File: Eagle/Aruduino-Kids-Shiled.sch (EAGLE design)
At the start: 20 parts

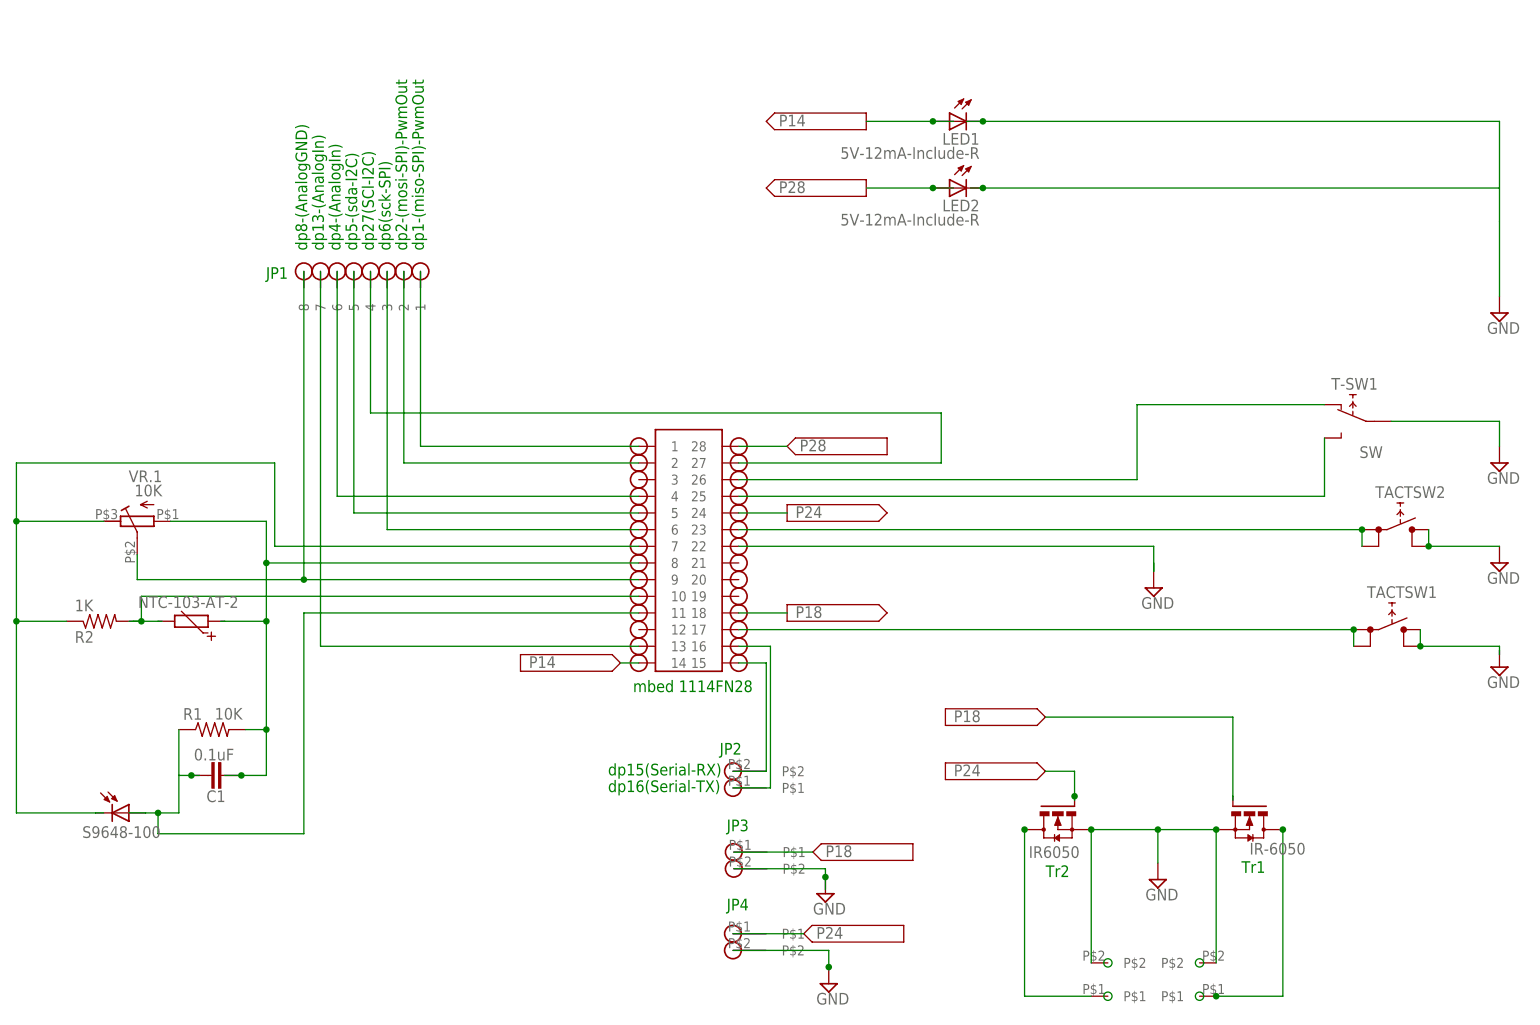
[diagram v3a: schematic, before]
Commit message: Final-P-ban
1st time
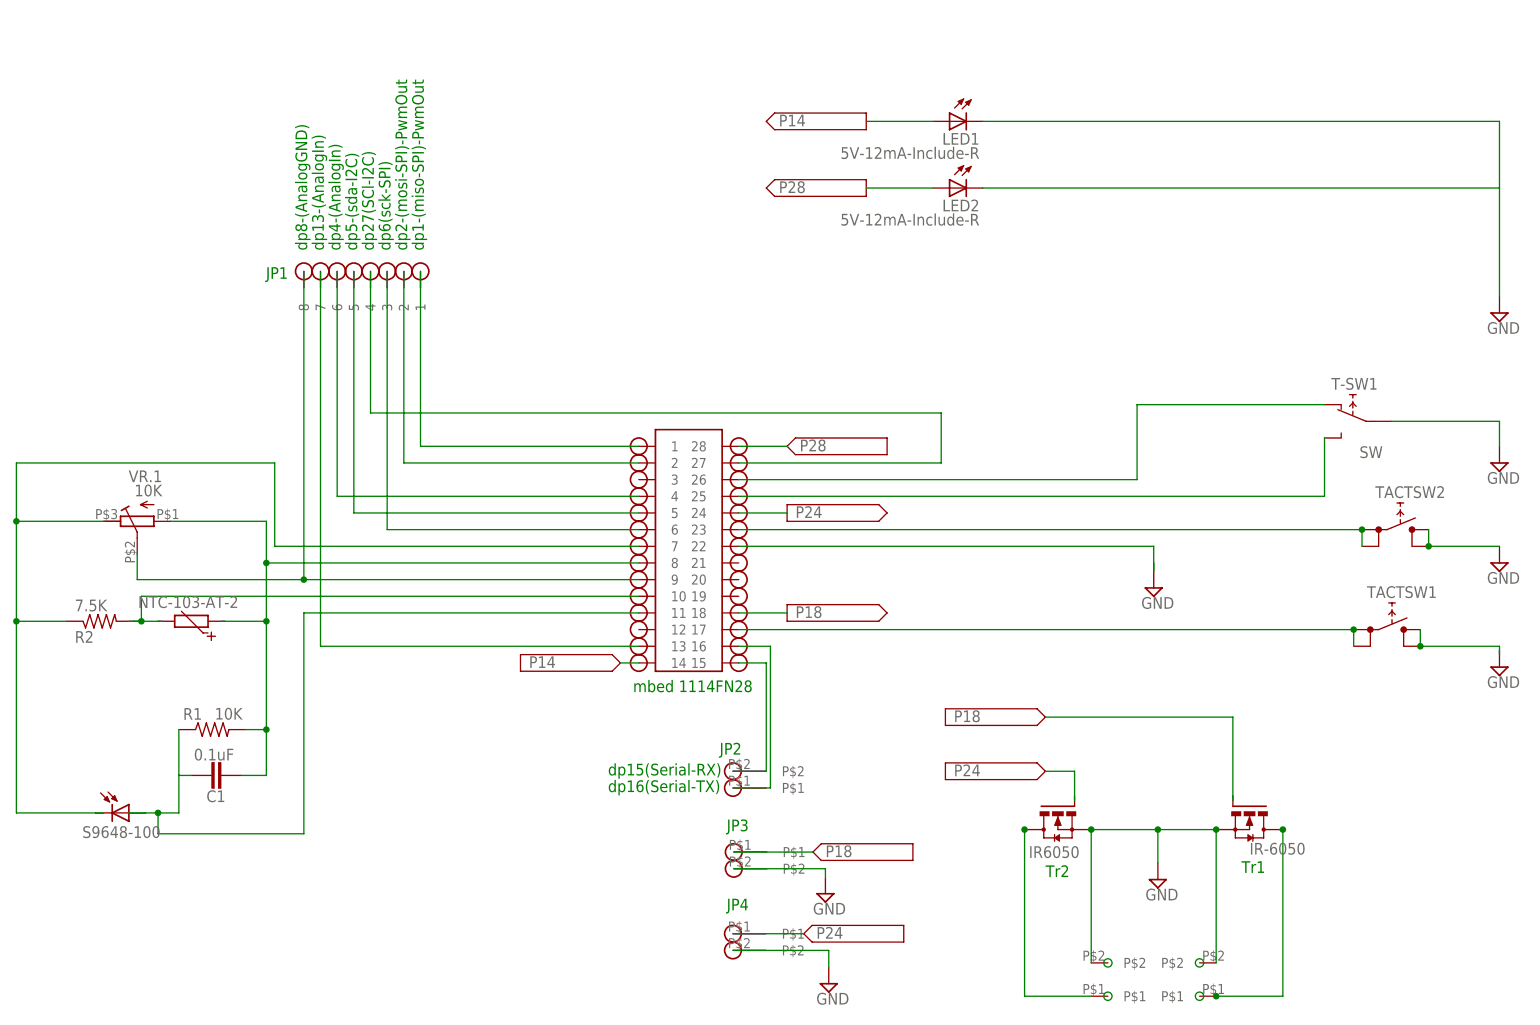
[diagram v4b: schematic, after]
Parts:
- R2: value 1K -> 7.5K
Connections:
- net GND renamed N$126
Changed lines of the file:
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@@
 <part name="SUPPLY12" library="supply2" deviceset="V&lt;--" device="" value="P18"/>
 <part name="SUPPLY13" library="supply2" deviceset="GND" device=""/>
-<part name="R2" library="Aruduino-Kids-Shiled" deviceset="R" device="" value="1K"/>
+<part name="R2" library="Aruduino-Kids-Shiled" deviceset="R" device="" value="7.5K"/>
 <part name="TACTSW2" library="Aruduino-Kids-Shiled" deviceset="TACT-SW" device=""/>
 <part name="TACTSW1" library="Aruduino-Kids-Shiled" deviceset="TACT-SW" device=""/>
@@
 </segment>
 <segment>
-<wire x1="203.2" y1="71.755" x2="200.025" y2="71.755" width="0.1524" layer="91"/>
 <pinref part="LED1" gate="G$1" pin="A"/>
 <wire x1="200.025" y1="71.755" x2="189.865" y2="71.755" width="0.1524" layer="91"/>
-<junction x="200.025" y="71.755"/>
 </segment>
 </net>
@@
 </segment>
 <segment>
-<wire x1="203.2" y1="61.595" x2="200.025" y2="61.595" width="0.1524" layer="91"/>
 <pinref part="LED2" gate="G$1" pin="A"/>
 <wire x1="200.025" y1="61.595" x2="189.865" y2="61.595" width="0.1524" layer="91"/>
-<junction x="200.025" y="61.595"/>
 </segment>
 </net>
@@
 <wire x1="98.425" y1="-20.955" x2="98.425" y2="-27.94" width="0.1524" layer="91"/>
 <junction x="98.425" y="-20.955"/>
-<wire x1="92.075" y1="-27.94" x2="94.615" y2="-27.94" width="0.1524" layer="91"/>
 <pinref part="C1" gate="G$1" pin="1"/>
 <wire x1="94.615" y1="-27.94" x2="98.425" y2="-27.94" width="0.1524" layer="91"/>
-<junction x="94.615" y="-27.94"/>
 <wire x1="91.44" y1="-4.445" x2="92.075" y2="-4.445" width="0.1524" layer="91"/>
 <wire x1="92.075" y1="-4.445" x2="98.425" y2="-4.445" width="0.1524" layer="91"/>
@@
 </segment>
 </net>
-<net name="GND" class="0">
+<net name="N$126" class="0">
 <segment>
 <pinref part="SUPPLY3" gate="GND" pin="GND"/>
@@
 </segment>
 <segment>
-<wire x1="286.385" y1="45.085" x2="286.385" y2="56.515" width="0.1524" layer="91"/>
+<wire x1="286.385" y1="45.085" x2="286.385" y2="61.595" width="0.1524" layer="91"/>
 <pinref part="SUPPLY9" gate="GND" pin="GND"/>
 <wire x1="286.385" y1="61.595" x2="286.385" y2="71.755" width="0.1524" layer="91"/>
-<wire x1="205.105" y1="71.755" x2="207.645" y2="71.755" width="0.1524" layer="91"/>
 <wire x1="207.645" y1="71.755" x2="286.385" y2="71.755" width="0.1524" layer="91"/>
-<wire x1="205.74" y1="61.595" x2="207.645" y2="61.595" width="0.1524" layer="91"/>
+<pinref part="LED1" gate="G$1" pin="C"/>
+<pinref part="LED2" gate="G$1" pin="C"/>
 <wire x1="207.645" y1="61.595" x2="286.385" y2="61.595" width="0.1524" layer="91"/>
-<wire x1="286.385" y1="61.595" x2="286.385" y2="56.515" width="0.1524" layer="91"/>
-<pinref part="LED1" gate="G$1" pin="C"/>
-<junction x="207.645" y="71.755"/>
-<pinref part="LED2" gate="G$1" pin="C"/>
-<junction x="207.645" y="61.595"/>
 </segment>
 <segment>
@@
 <wire x1="184.15" y1="-54.61" x2="184.15" y2="-57.15" width="0.1524" layer="91"/>
 <pinref part="SUPPLY10" gate="GND" pin="GND"/>
-<junction x="184.15" y="-57.15"/>
 <pinref part="U$9" gate="G$1" pin="P$2"/>
 </segment>
@@
 <wire x1="183.642" y1="-42.164" x2="183.642" y2="-43.434" width="0.1524" layer="91"/>
 <pinref part="SUPPLY13" gate="GND" pin="GND"/>
-<wire x1="183.642" y1="-43.434" x2="183.642" y2="-45.339" width="0.1524" layer="91"/>
-<junction x="183.642" y="-43.434"/>
 </segment>
 </net>
@@
 <wire x1="221.615" y1="-27.305" x2="217.17" y2="-27.305" width="0.1524" layer="91"/>
 <pinref part="U$5" gate="G$1" pin="G"/>
-<junction x="221.615" y="-31.115"/>
 </segment>
 <segment>
@@
 <wire x1="81.915" y1="-36.83" x2="81.915" y2="-33.655" width="0.1524" layer="91"/>
 <junction x="81.915" y="-33.655"/>
-<wire x1="88.265" y1="-27.94" x2="86.995" y2="-27.94" width="0.1524" layer="91"/>
 <pinref part="C1" gate="G$1" pin="2"/>
 <wire x1="86.995" y1="-27.94" x2="85.09" y2="-27.94" width="0.1524" layer="91"/>
-<junction x="86.995" y="-27.94"/>
 <pinref part="U$1" gate="G$1" pin="11"/>
 </segment>
@@
 </sheet>
 </sheets>
+<errors>
+</errors>
 </schematic>
 </drawing>

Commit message: Test-Sample-Build
Jet-PCB
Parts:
- LED1: value 5V-12mA-Include-R -> I-06245-R
- LED2: value 5V-12mA-Include-R -> I-06245-G
- T-SW1: value SW -> P-00300
- TACTSW1: value (none) -> P-03646-B
- TACTSW2: value (none) -> P-03646-R
- TB1, TB2: value 2A -> P-01306
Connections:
- net N$4 renamed 3.3V
- removed net N$126: LED1.C, LED2.C, T-SW1.2COM, TACTSW1.2, TACTSW1.4, TACTSW2.2, TACTSW2.4, TB1.P$2, TB2.P$2, U$1.22, U$10.P$2, U$4.S, U$5.S, U$9.P$2
- removed net N$6: 0-50C.1, C1.1, R1.2, U$1.8, VR.1.A
- new net A-GND: 0-50C.1, C1.1, R1.2, U$1.8, U$3.8, VR.1.A
- new net GND: LED1.C, LED2.C, T-SW1.2COM, TACTSW1.2, TACTSW1.4, TACTSW2.2, TACTSW2.4, TB1.P2, TB2.P2, U$1.22, U$10.P2, U$4.S, U$5.S, U$9.P2
- net N$21: now also TB2.P1; no longer TB2.P$1
- net N$22: now also TB1.P1; no longer TB1.P$1
- net N$26: now also U$6.P1; no longer U$6.P$1
- net N$27: now also U$6.P2; no longer U$6.P$2
- net N$8: no longer U$3.8
- net P18: now also U$10.P1; no longer U$10.P$1
- net P24: now also U$9.P1; no longer U$9.P$1
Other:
- note added: "C-03785"
- note added: "C-05779 (TP2,TP3,TP4)"
- note added: "I-02426"
- note added: "P-01306"
- note added: "P-06113"
- note added: "P-06165"
- note added: "P-07258"
- note added: "P1"
- note added: "P2"
- note added: "R-25103"
- note added: "R-25752"
- note added: "TP1"
- note added: "TP2"
- note added: "TP3"
- note added: "TP4"
- note removed: "JP1"
- note removed: "JP2"
- note removed: "JP3"
- note removed: "JP4"
- moved on the sheet: C1, LED1, LED2, R1, R2, T-SW1, TACTSW1, TACTSW2, VR.1
